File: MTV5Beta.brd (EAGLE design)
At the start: 85 x 70 mm, 99 parts, among them IC1 OPA2365U, IC2 MCP1700-3302, IC3 MCP1700-3302, J1 MICROUSB, J2 SWDPORT, U1 STM32F405RGT6, U2 ADS8330IB, U3 MX66L51235FZ2I-10G

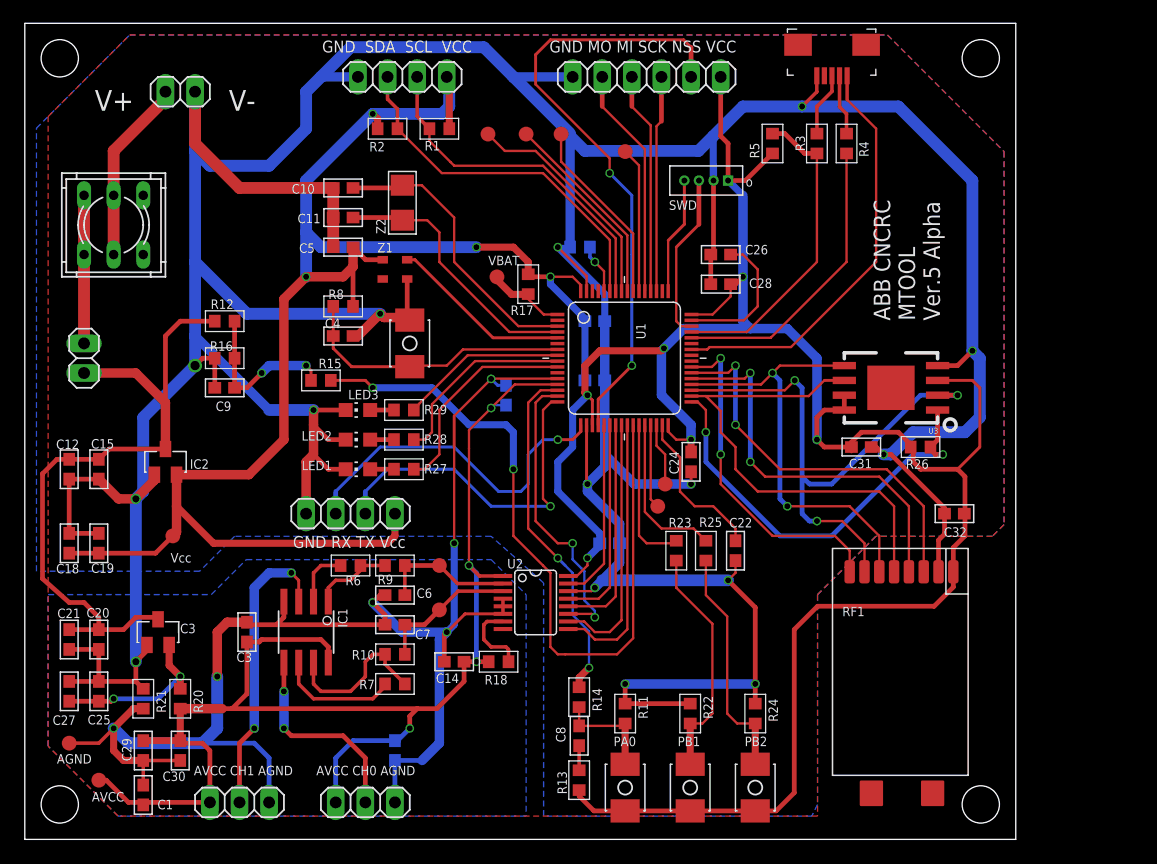
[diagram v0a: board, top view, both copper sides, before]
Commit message: Upload files
Upload files
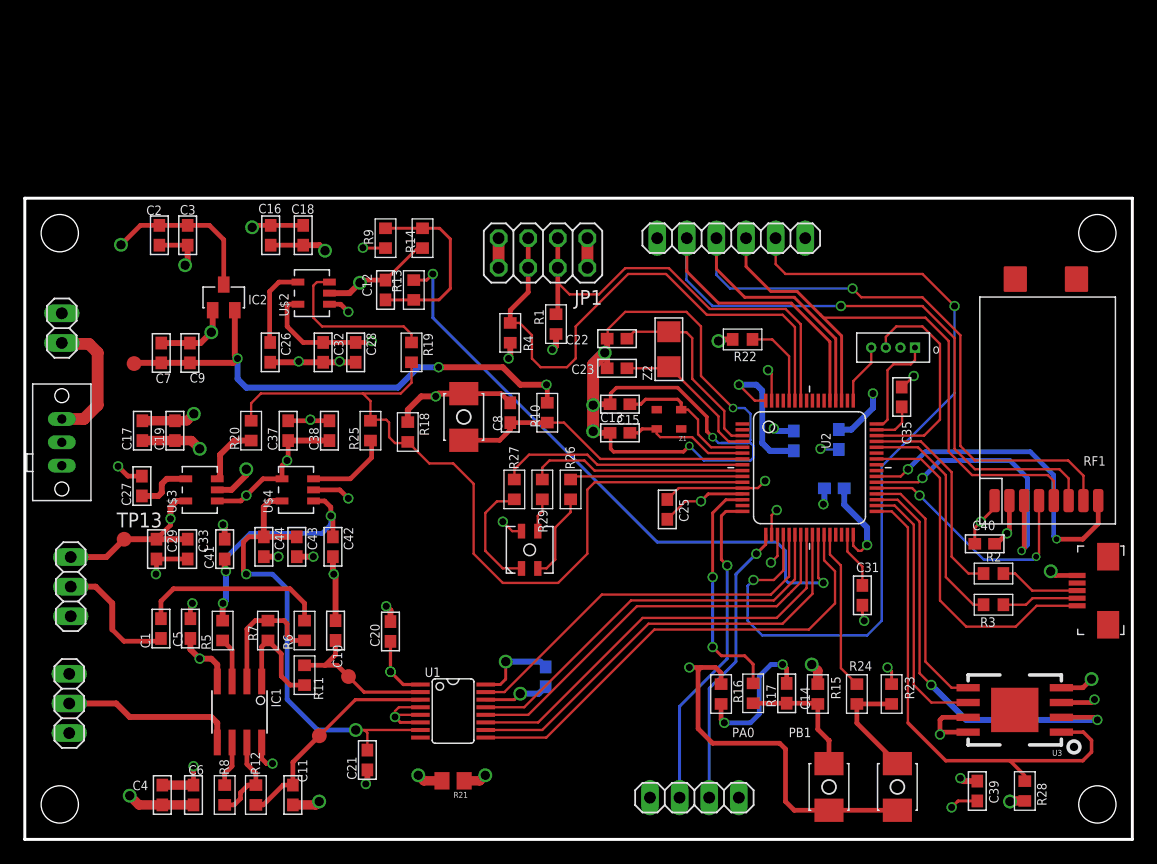
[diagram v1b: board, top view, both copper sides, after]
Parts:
- removed IC3: MCP1700-3302, LDO:SOT23
- removed JP7: (no value), pinhead:1X06
- removed LED1: red, led:CHIP-LED0805
- removed LED2: green, led:CHIP-LED0805
- removed LED3: blue, led:CHIP-LED0805
- removed PB4: PB, switch-misc:BUTTON
- removed S1: 9077-2, switch-misc:9077-2
- removed TP10, TP11, TP12, TP2, TP5, TP6, TP7, TP8, TP9: TPB1,27, testpad:B1,27
- added C33, C34, C36, C38, C39, C40, C42, C44: 0.1uF, rcl:C0603
- added C35, C37, C41, C43: 2.2uF, rcl:C0603
- added TP13: TPB1,27, testpad:B1,27
- added U$1: 3P-SW, EF_Lib:3P-2-SW
- added U$2, U$3: TPS73433, EF_Lib:SOT-5
- added U$4: REF2033, EF_Lib:SOT-5
- added U$5: LED-RGB, EF_Lib:LED-3228
- C10, C11: value 6.8pF -> 470pF
- C12, C14, C18, C20, C25: value 10uF -> 0.1uF
- C13: value 1uF -> 20pF
- C15: value 0.1uF -> 20pF
- C16, C17: value 0.1uF -> 10uF
- C2: value 1uF -> 10uF
- C22: value 2.2uF -> 6.8pF
- C23: value 1uF -> 6.8pF
- C27, C28: value 0.1uF -> 2.2uF
- C29: value 10uF -> 2.2uF
- C3, C32, C9: value 1uF -> 0.1uF
- C31: value 1uF -> 2.2uF
- C4: value 0.1uF -> 1uF
- C6: value 470pF -> 1uF
- C7: value 470pF -> 10uF
- JP1: device pinhead:1X04 -> pinhead:2X04
- JP2: device pinhead:1X04 -> pinhead:1X02
- JP3: device pinhead:1X03 -> pinhead:1X04
- JP5: device pinhead:1X02 -> pinhead:1X03
- JP6: device pinhead:1X02 -> pinhead:1X06
- R10: value 20 -> 10k
- R11, R12, R16, R24: value 100k -> 100
- R13: value 100 -> 10k
- R14: value 220 -> 1M
- R15, R23: value 100 -> 100k
- R17: value 0 -> 100
- R18: value 0 -> 100k
- R19: value 10k -> 100
- R2: value 2k -> 22
- R20: value 1uH -> 100
- R21: device rcl:R0603 -> rcl:R0805
- R22: value 100k -> 10k
- R26: value 10k -> 1k
- R27, R29: value 470 -> 1k
- R28: value 470 -> 10k
- R4: value 22 -> 2k
- R5: value 2k -> 1k
- R6: value 20 -> 1k
- R7: value 20 -> 50k
- R8: value 10k -> 20
- R9: value 20 -> 1M
- U1: value STM32F405RGT6 -> ADS8330IB; device EF_Lib:LQFP64 -> EF_Lib:TSSOP16
- U2: value ADS8330IB -> STM32F405RGT6; device EF_Lib:TSSOP16 -> EF_Lib:LQFP64
- Z1: value ASE -> Z-4P; device crystal:ASE -> EF_Lib:ASE
- moved R2 64.5 mm to (83.1, 22.8)
- moved R5 63.0 mm to (17.0, 17.9)
- moved R28 61.2 mm to (85.8, 4.15), turned to 90 degrees
- moved JP6 56.5 mm to (60.6, 51.6), turned to 180 degrees
- moved C32 55.9 mm to (25.6, 41.8), turned to 270 degrees
- moved JP5 53.3 mm to (3.81, 11.7), turned to 270 degrees
- moved R16 51.4 mm to (59.7, 12.5), turned to 90 degrees
- moved J1 51.3 mm to (92.1, 21.4), turned to 180 degrees
- moved C25 51.2 mm to (55.1, 28.3)
- moved R15 50.4 mm to (68.0, 12.5), turned to 270 degrees
- moved C11 49.7 mm to (23.0, 3.81), turned to 270 degrees
- moved C2 48.6 mm to (11.5, 51.8), flipped to the top, turned to 270 degrees
- moved C15 45.0 mm to (51.0, 37.3), turned to 180 degrees
- moved R13 44.4 mm to (33.4, 47.1)
- moved R8 43.1 mm to (17.1, 3.81), turned to 90 degrees
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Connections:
- removed net N$22: R14.1, U1.14
- removed net N$24: R17.1, TP7.TP, U1.1
- removed net N$28: TP6.TP, U1.57
- removed net N$30: TP8.TP, U1.56
- removed net N$31: TP9.TP, U1.55
- removed net N$32: TP10.TP, U1.54
- removed net N$34: TP11.TP, U1.29
- removed net N$35: TP12.TP, U1.30
- removed net PB1: R23.1, U1.27
- new net LDO_EN: R18.2, R19.2, R20.2, R25.2, U2.11
- new net N$36: C27.1, U$3.4
- new net N$37: IC1.1, R11.2, R7.1
- new net N$38: IC1.3, R5.1
- new net N$40: C1.2, R6.2
- new net PA0: R17.1, U2.14
- new net VBIAS: C41.1, C42.1, R5.2, U$4.1
- new net VCC_DEV: C28.1, C30.1, C32.1, C39.1, C40.1, JP1.1, JP1.2, JP3.1, JP6.1, R1.2, R28.1, R4.2, RF1.1, U$2.5, U$5.2, U1.16, U3.3, U3.7, U3.8
- new net VREF: C21.2, C43.1, C44.1, U$4.5, U1.7
- net ADS_CH0: now also C11.1, R12.1, U1.3; no longer C7.1, R10.1, U2.3
- net ADS_CH1: now also C10.1, R11.1, U1.2; no longer C6.1, R9.1, U2.2
- net AD_CONVST: now also U1.9, U2.27; no longer U1.25, U2.9
- net AD_CS: now also U1.11, U2.24; no longer U1.15, U2.11
- net AD_INT: now also U1.10, U2.25; no longer U1.24, U2.10
- net AGND: now also C10.2, C11.2, C17.2, C19.2, C20.2, C21.1, C27.2, C33.2, C37.2, C38.2, C4.1, C41.2, C42.2, C43.2, C44.2, C5.1, C6.1, JP5.3, U$3.2, U$4.2, U1.4, U1.5, U1.6; no longer C1.1, C13.2, C14.1, C2.1, C3.1, C30.2, C6.2, C7.2, JP3.3, TP5.TP, U1.12, U2.4, U2.5, U2.6
- net AVCC: now also C20.1, C33.1, C4.2, C5.2, C6.2, JP5.1, TP13.TP, U$3.5, U1.1; no longer C1.2, C13.1, C14.2, C2.2, C3.2, C30.1, JP3.1, R18.2, R20.2, TP2.TP, U1.13, U2.1
- net BAT_IN: now also R13.1, U2.26; no longer R15.1, U1.26
- net FLASH_CS: now also R28.2, U2.33; no longer R26.2, U1.33
- net GND: now also C13.1, C2.2, C24.2, C28.2, C3.2, C30.2, C34.1, C35.2, C36.1, C39.2, C40.2, C7.2, C8.2, JP1.7, JP1.8, JP2.2, JP3.4, JP6.6, R14.1, R15.1, R18.1, R23.1, U$2.2, U1.14, U2.12, U2.18, U2.63; no longer C10.2, C11.2, C17.2, C19.2, C20.2, C21.2, C24.1, C27.2, C28.1, C4.2, C5.2, IC3.1, JP1.4, JP2.4, JP5.2, JP7.6, LED1.C, LED2.C, LED3.C, R11.1, R16.1, R19.1, R24.1, U1.18, U1.63, U2.14, Z1.2
- net I2C1_SCL: now also JP1.3, JP1.4, U2.58; no longer JP1.2, U1.58
- net I2C1_SDA: now also JP1.5, JP1.6, R4.1, U2.59; no longer JP1.3, R2.1, U1.59
- net LED_BLUE: now also R26.2, U2.10; no longer R27.2, U1.10
- net LED_GREEN: now also R29.1, U2.9; no longer R28.2, U1.9
- net LED_RED: now also R27.2, U2.8; no longer R29.2, U1.8
- net N$1: now also R22.2, U2.60; no longer R19.2, U1.60
- net N$10: now also R25.1, U$4.3; no longer U1.5, Z1.3
- net N$11: now also C35.1, U2.47; no longer C26.1, U1.47
- net N$12: now also JP5.2; no longer JP4.2
- net N$13: now also R12.2, R8.1; no longer R10.2, R7.1
- net N$14: now also C12.1, R13.2, R14.2, R9.1; no longer C9.1, R12.1, R15.2, R16.2
- net N$15: now also R8.2; no longer R7.2
- net N$16: now also C26.1, U$2.4; no longer JP6.2, S1.1, S1.4
- net N$17: now also JP2.1, U$1.P$3; no longer JP5.1, S1.2, S1.5
- net N$18: now also C14.1, R16.1; no longer C8.1, R13.1
- net N$19: now also U$5.1; no longer LED1.A
- net N$2: now also R3.1; no longer R4.1
- net N$20: now also C14.2, R15.2, R17.2; no longer C8.2, R11.2, R14.2
- net N$21: now also R26.1, U$5.3; no longer LED2.A, R28.1
- net N$23: now also R29.2, U$5.4; no longer LED3.A, R29.1
- net N$25: now also C22.1, U2.3; no longer C10.1, U1.3
- net N$26: now also C23.1, U2.4; no longer C11.1, U1.4
- net N$27: now also R24.2; no longer R22.2
- net N$29: now also R20.1, U$3.3; no longer PB4.1, R24.2, R25.2
- net N$3: now also R2.1; no longer R3.1
- net N$4: now also C31.1, U2.31; no longer C22.1, U1.31
- net N$41: now also IC1.2, R6.1, R7.2; no longer R18.1, U2.7
- net N$5: now also C15.1, U2.5, Z1.1; no longer IC1.1, R6.1, R9.2
- net N$6: now also C8.1, R10.1, U2.7; no longer C4.1, R8.1, U1.7
- net N$7: now also R19.1, U$2.3; no longer C25.1, C27.1, IC3.2, R20.1
- net N$8: now also C13.2, U2.6, Z1.3; no longer IC1.2, R6.2
- net N$9: now also C1.1, JP4.2; no longer IC1.3, JP3.2
- net NRF_CE: now also U2.38; no longer U1.38
- net NRF_CS: now also U2.37; no longer U1.37
- net NRF_INT: now also U2.39; no longer U1.39
- net PB2: now also R24.1, U2.28; no longer R25.1, U1.28
- net SPI1_MISO: now also U1.13, U2.22; no longer U1.22, U2.13
- net SPI1_MOSI: now also U1.12, U2.23; no longer U1.23, U2.12
- net SPI1_SCK: now also U1.15, U2.21; no longer U1.21, U2.15
- net SPI2_MISO: now also U2.35; no longer RF1.7, U1.35
- net SPI2_MOSI: now also U2.36; no longer RF1.6, U1.36
- net SPI2_SCK: now also U2.34; no longer RF1.5, U1.34
- net SPI3_MISO: now also JP6.4, RF1.7, U2.52; no longer JP7.4, U1.52
- net SPI3_MOSI: now also JP6.5, RF1.6, U2.53; no longer JP7.5, U1.53
- net SPI3_NSS: now also JP6.2, U2.20; no longer JP7.2, U1.20
- net SPI3_SCK: now also JP6.3, RF1.5, U2.51; no longer JP7.3, U1.51
- net SWCLK: now also U2.49; no longer U1.49
- net SWDIO: now also U2.46; no longer U1.46
- net UART2_RX: now also JP3.3, U2.17; no longer JP2.3, U1.17
- net UART2_TX: now also JP3.2, U2.16; no longer JP2.2, U1.16
- net USB_DM: now also R3.2, U2.44; no longer R4.2, U1.44
- net USB_DP: now also R2.2, U2.45; no longer R3.2, R5.2, U1.45
- net VBUS: now also U2.42; no longer U1.42
- net VCC: now also C24.1, C25.1, C34.2, C36.2, C7.1, C9.1, R10.2, R16.2, U2.1, U2.13, U2.19, U2.32, U2.48, U2.64; no longer C16.1, C17.1, C18.1, C19.1, C23.1, C24.2, C28.2, C31.1, C32.1, C5.1, JP1.1, JP2.1, JP7.1, PB4.2, R1.2, R13.2, R17.2, R2.2, R26.1, R5.1, R8.2, RF1.1, U1.19, U1.32, U1.48, U1.64, U2.16, U3.3, U3.7, U3.8, Z1.4
- net VIN: now also C16.1, C17.1, C18.1, C19.1, C2.1, C3.1, C37.1, C38.1, R9.2, U$1.P$2, U$2.1, U$3.1, U$4.4; no longer C12.1, C15.1, C20.1, C21.1, IC3.3, JP6.1, R12.2
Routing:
- net VCC_DEV: track 0.00 -> 222.7 mm, vias 0 -> 10
- net VCC: track 338.8 -> 206.3 mm, vias 10 -> 9
- net AGND: track 131.7 -> 203.0 mm, vias 6 -> 17
- net LDO_EN: track 0.00 -> 69.2 mm
- net SPI3_MOSI: track 19.9 -> 73.6 mm, vias 0 -> 1
- net SPI3_MISO: track 19.0 -> 70.1 mm, vias 0 -> 1
- net VIN: track 58.2 -> 105.3 mm, vias 0 -> 7
- net VREF: track 0.00 -> 40.6 mm, vias 0 -> 2
- net SPI3_SCK: track 18.6 -> 51.8 mm
- net N$22: track 29.9 -> 0.00 mm, vias 2 -> 0
- net VBIAS: track 0.00 -> 21.9 mm, vias 0 -> 3
- net AVCC: track 115.0 -> 93.5 mm, vias 4 -> 6
- net PA0: track 0.00 -> 20.3 mm, vias 0 -> 2
- net N$28: track 19.8 -> 0.00 mm
- net SPI2_SCK: track 41.5 -> 22.9 mm
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- added copper zone on layer 2, net AGND
- added copper zone on layer 2, net GND
- removed copper zone on layer 16, net AGND
- removed copper zone on layer 16, net GND
- removed copper zone on layer 1, net N$33
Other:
- board size 85 x 70 mm -> 95 x 55 mm
- board text removed: "ABB CNCRC MTOOL Ver.5 Alpha"
- board text removed: "AGND"
- board text removed: "AVCC"
- board text removed: "AVCC CH0 AGND"
- board text removed: "AVCC CH1 AGND"
- board text removed: "GND MO MI SCK NSS VCC"
- board text removed: "GND RX TX Vcc"
- board text removed: "GND SDA SCL VCC"
- board text removed: "PB2"
- board text removed: "SWD"
- board text removed: "V+"
- board text removed: "V-"
- board text removed: "VBAT"
- board text removed: "Vcc"

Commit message: v1.0 finished
sch ERC OK!
pcb DRC OK!
gerb export OK!
PDF export OK!
need adding BOM
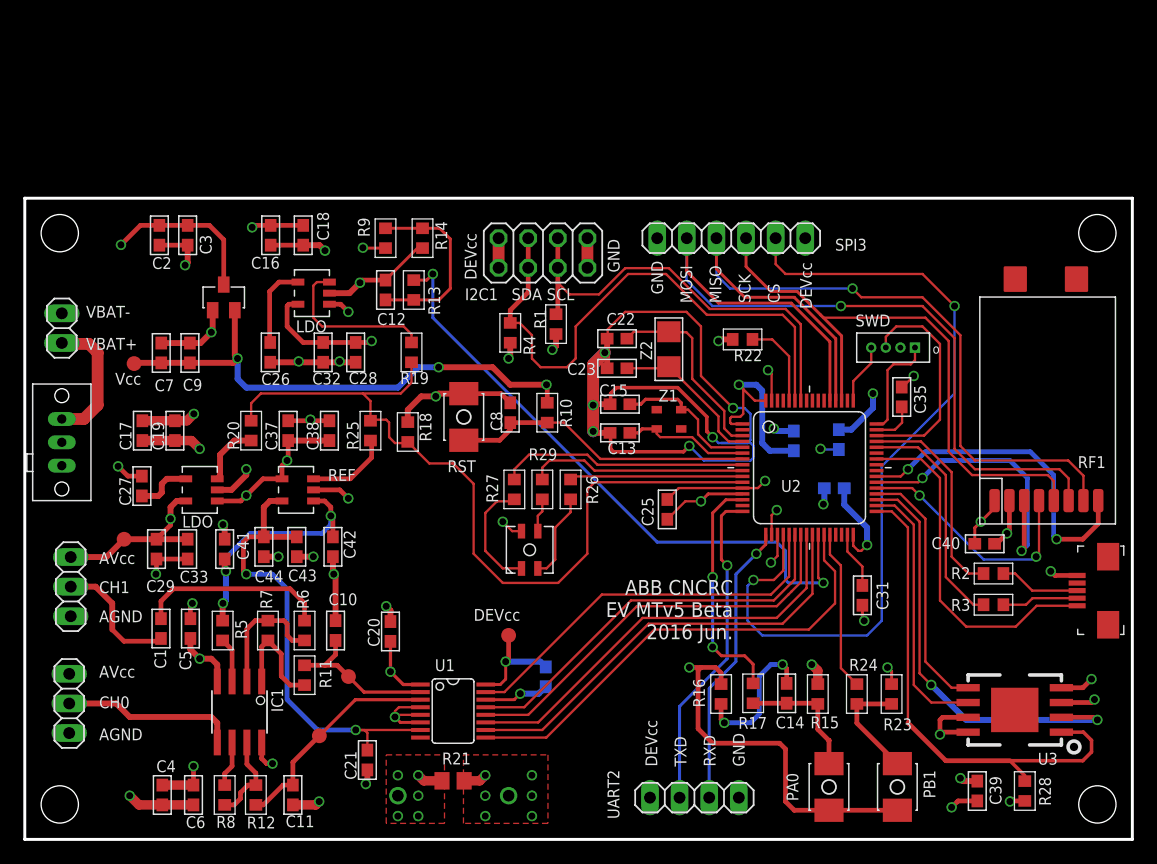
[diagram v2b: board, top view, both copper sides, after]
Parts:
- added TP2: TPB1,27, testpad:B1,27
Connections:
- net VCC_DEV: now also TP2.TP
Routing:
- net VCC: track 206.3 -> 211.7 mm
- net VCC_DEV: track 222.7 -> 225.1 mm
- net AGND: track 203.0 -> 204.8 mm, vias 17 -> 22
- net GND: track 424.3 -> 425.7 mm, vias 30 -> 35
- net AVCC: vias 6 -> 5
- added copper zone on layer 1, net AGND
- added copper zone on layer 1, net GND
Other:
- board text added: "ABB CNCRC EV MTv5 Beta 2016 Jun."
- board text added: "AGND"
- board text added: "AVcc"
- board text added: "CH0"
- board text added: "CH1"
- board text added: "CS"
- board text added: "DEVcc"
- board text added: "GND"
- board text added: "I2C1"
- board text added: "LDO"
- board text added: "MISO"
- board text added: "MOSI"
- board text added: "REF"
- board text added: "RST"
- board text added: "RXD"
- board text added: "SCK"
- board text added: "SDA SCL"
- board text added: "SPI3"
- board text added: "SWD"
- board text added: "TXD"
- board text added: "UART2"
- board text added: "VBAT+"
- board text added: "VBAT-"
- board text added: "Vcc"
